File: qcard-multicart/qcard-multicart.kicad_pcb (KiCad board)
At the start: 2 copper layers, 1 part, among them U1 MX29LV640EBTI-70G

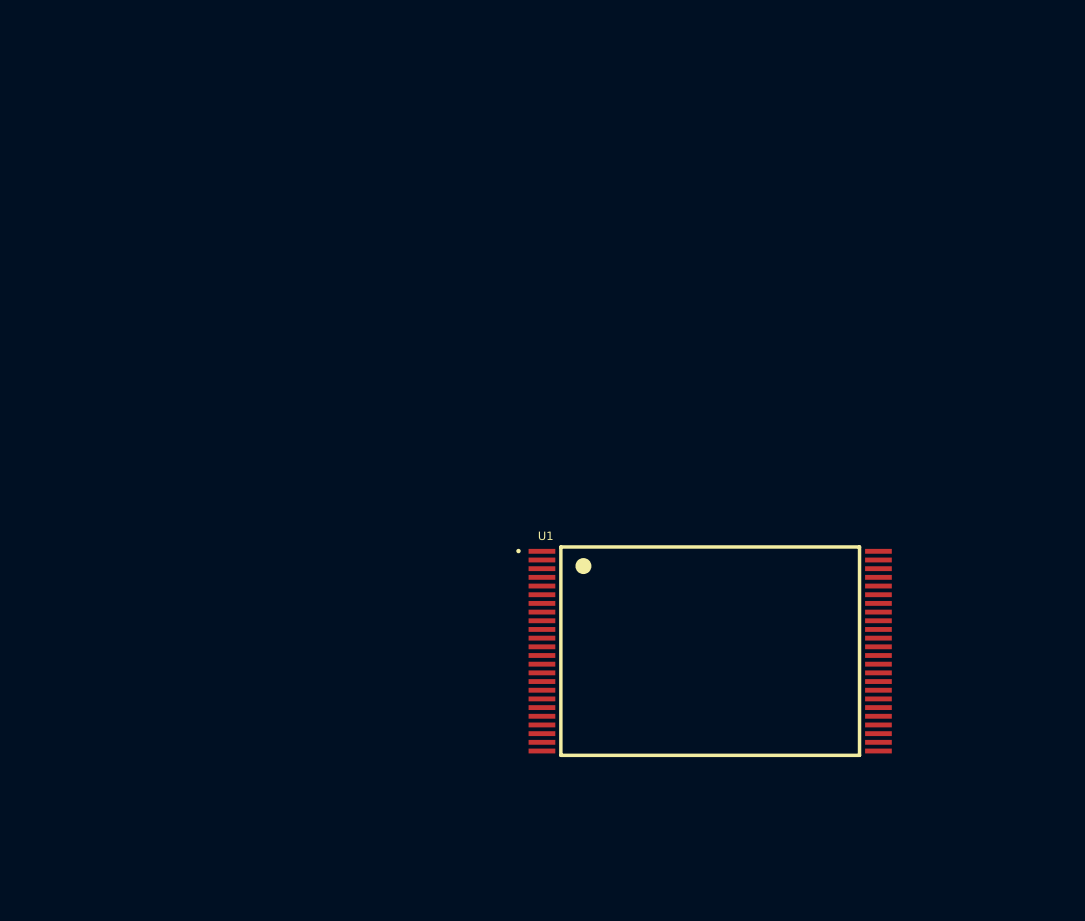
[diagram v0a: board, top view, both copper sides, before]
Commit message: First pass at multicart
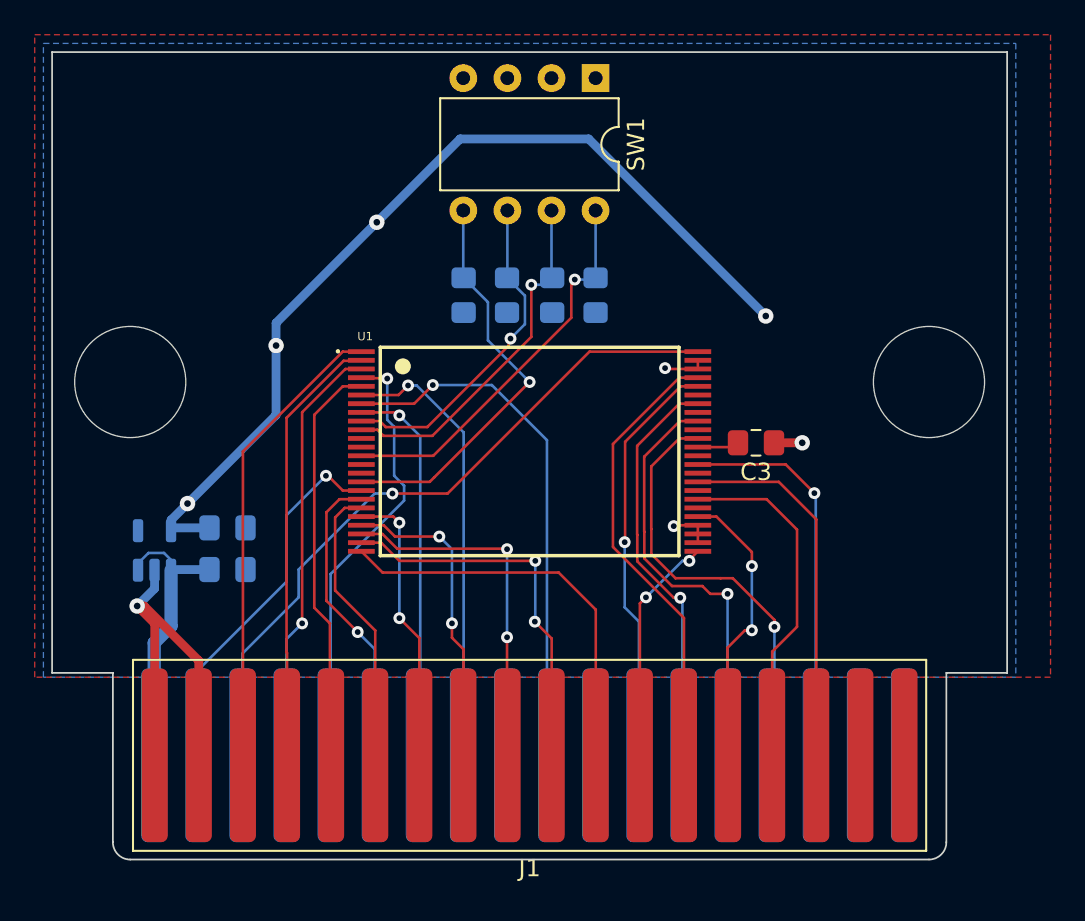
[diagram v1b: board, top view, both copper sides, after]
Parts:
- added C1: 1uF, Capacitor_SMD:C_0805_2012Metric_Pad1.18x1.45mm_HandSolder, B.Cu at (79.6, 64.8)
- added C2: 1uF, Capacitor_SMD:C_0805_2012Metric_Pad1.18x1.45mm_HandSolder, B.Cu at (79.6, 62.4)
- added C3: 100pF, Capacitor_SMD:C_0805_2012Metric_Pad1.18x1.45mm_HandSolder, F.Cu at (110.0, 57.5)
- added J1: Conn_02x18_Top_Bottom, reb-edge:REB_EdgeConnector_36pin, F.Cu at (97.0, 75.5)
- added R1: R, Resistor_SMD:R_0805_2012Metric_Pad1.20x1.40mm_HandSolder, B.Cu at (93.2, 49.0)
- added R2: R, Resistor_SMD:R_0805_2012Metric_Pad1.20x1.40mm_HandSolder, B.Cu at (95.7, 49.0)
- added R3: R, Resistor_SMD:R_0805_2012Metric_Pad1.20x1.40mm_HandSolder, B.Cu at (98.3, 49.0)
- added R4: R, Resistor_SMD:R_0805_2012Metric_Pad1.20x1.40mm_HandSolder, B.Cu at (100.8, 49.0)
- added REF**: MountingHole_6.4mm_M6, MountingHole:MountingHole_6.4mm_M6, F.Cu at (74.0, 54.0)
- added REF**: MountingHole_6.4mm_M6, MountingHole:MountingHole_6.4mm_M6, F.Cu at (120.0, 54.0)
- added SW1: SW_DIP_x04, Package_DIP:DIP-8_W7.62mm, F.Cu at (100.8, 36.5)
- added U2: MIC5365-3.3YD5, Package_TO_SOT_SMD:SOT-23-5, B.Cu at (75.4, 63.7)
- moved U1 15.5 mm to (97.0, 58.0)
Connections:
- U1 pad 30: +3.3V -> unconnected-(U1-Pad30)
- U1 pad 32: +3.3V -> unconnected-(U1-Pad32)
- U1 pad 34: +3.3V -> unconnected-(U1-Pad34)
- U1 pad 36: +3.3V -> unconnected-(U1-Pad36)
- U1 pad 39: +3.3V -> unconnected-(U1-Pad39)
- U1 pad 41: +3.3V -> unconnected-(U1-Pad41)
- U1 pad 43: +3.3V -> unconnected-(U1-Pad43)
- U1 pad 47: +3.3V -> GND
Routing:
- net +3.3V: track 0.00 -> 56.0 mm, vias 0 -> 4
- net /A17: track 0.00 -> 40.2 mm, vias 0 -> 1
- net /A10: track 0.00 -> 30.7 mm, vias 0 -> 1
- net GND: track 0.00 -> 28.2 mm, vias 0 -> 4
- net /A16: track 0.00 -> 26.7 mm
- net /A0: track 0.00 -> 26.1 mm
- net /A11: track 0.00 -> 25.9 mm, vias 0 -> 1
- net /A15: track 0.00 -> 25.1 mm
- net /D4: track 0.00 -> 24.9 mm, vias 0 -> 1
- net /D5: track 0.00 -> 24.7 mm, vias 0 -> 1
- net /A14: track 0.00 -> 24.6 mm, vias 0 -> 1
- net /A13: track 0.00 -> 24.6 mm, vias 0 -> 1
- net /D7: track 0.00 -> 23.9 mm, vias 0 -> 1
- net /D6: track 0.00 -> 23.7 mm, vias 0 -> 1
- net Net-(R1-Pad1): track 0.00 -> 23.5 mm, vias 0 -> 1
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- added copper zone on F.Cu, net +3.3V
- added copper zone on B.Cu, net GND
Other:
- board outline added: 55 x 46.5 mm
